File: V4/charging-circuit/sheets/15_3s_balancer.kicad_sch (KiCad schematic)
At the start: 29 parts, among them Q12 AO4892, Q13 BSS84, SW2 TS-1088R-02026, U16 NTC10K/0805/F, U20 BQ76920PW

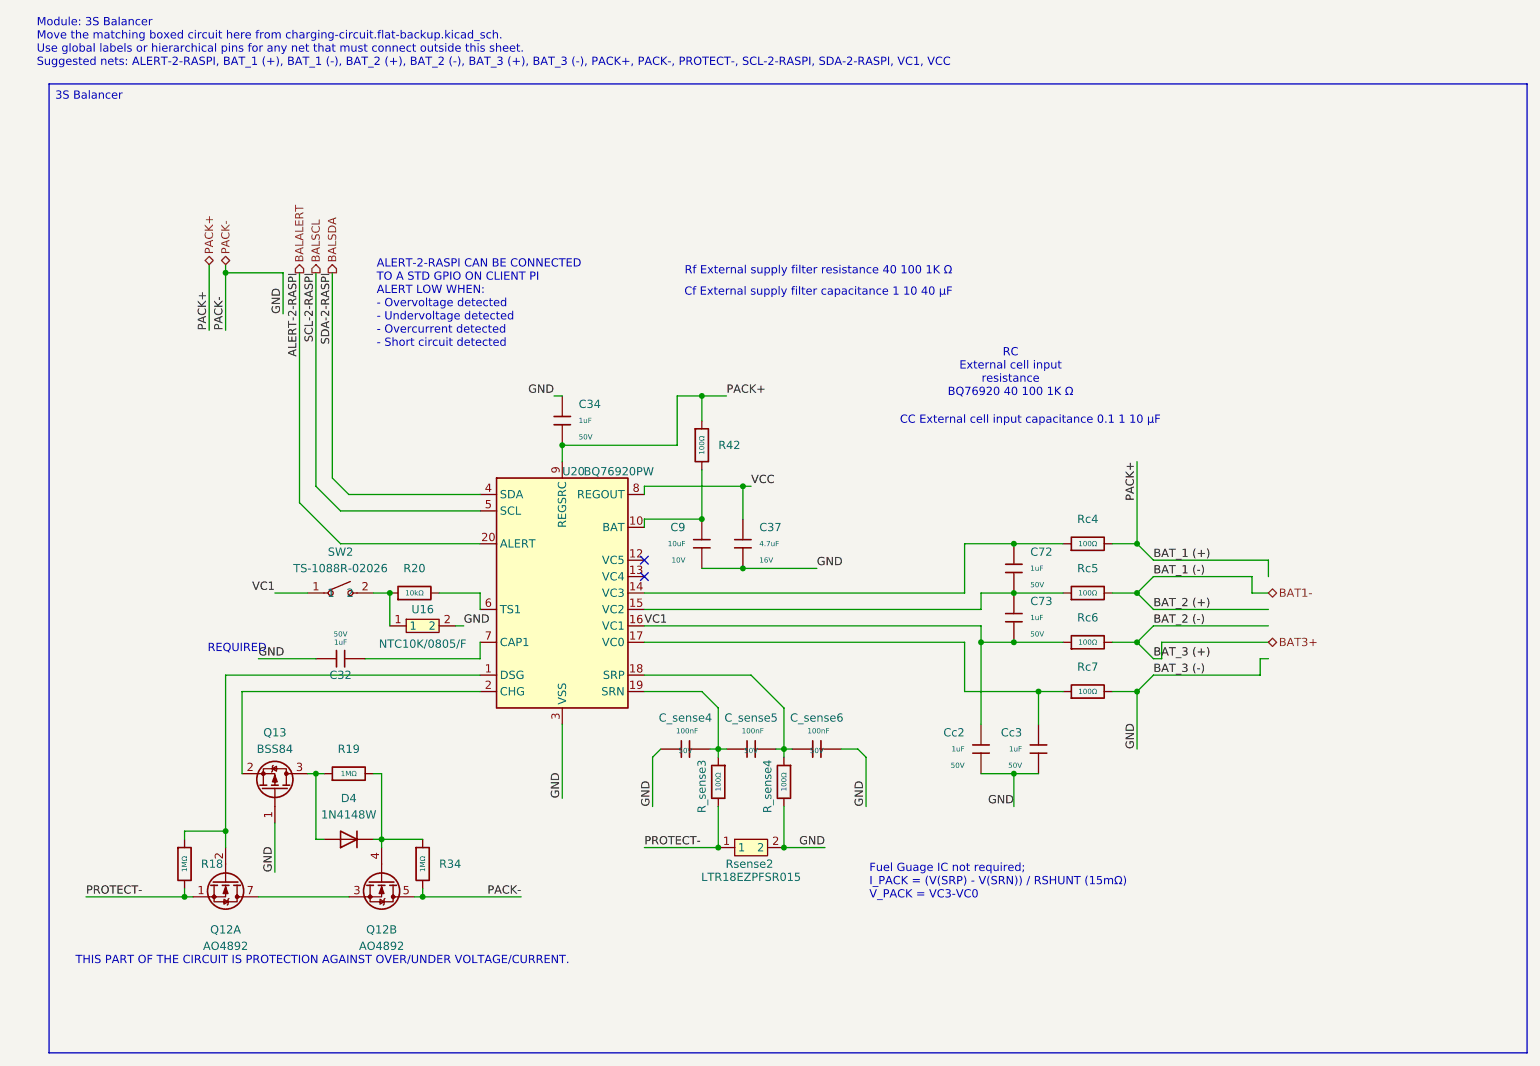
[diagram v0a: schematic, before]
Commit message: schem
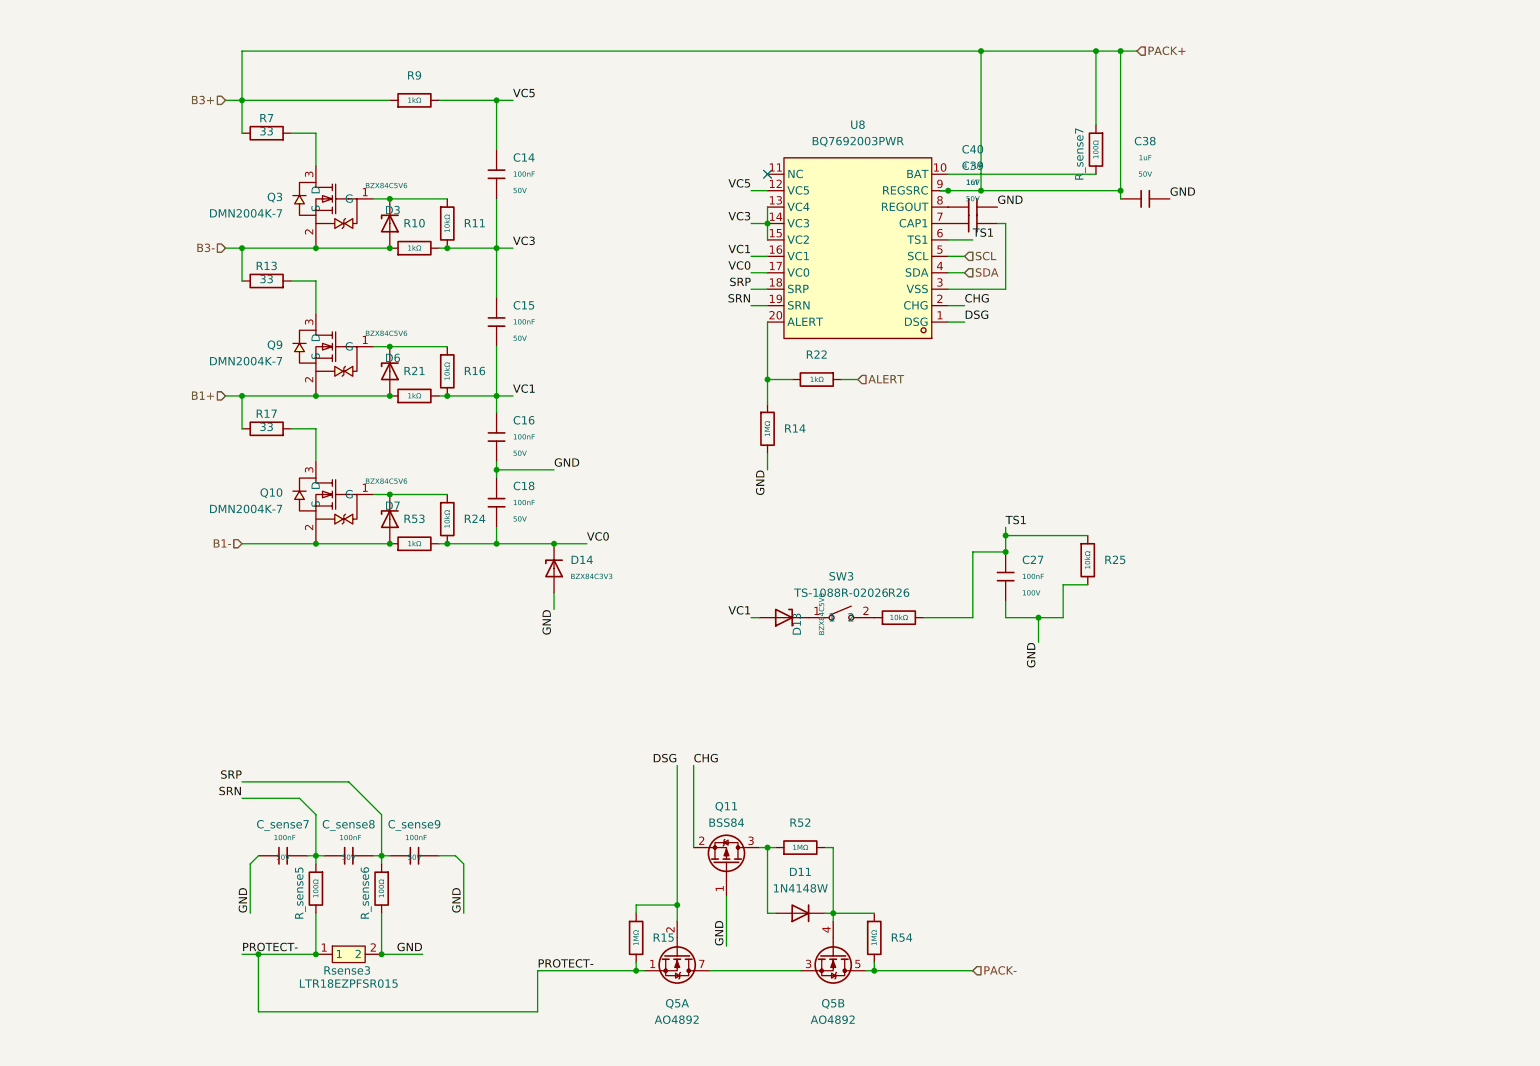
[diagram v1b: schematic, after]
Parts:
- removed C32: 1uF, PCM_JLCPCB:C_1206, symbol PCM_JLCPCB-Capacitors:1206,1uF
- removed C34, C72, C73, Cc2, Cc3: 1uF, PCM_JLCPCB:C_0603, symbol PCM_JLCPCB-Capacitors:0603,1uF
- removed C37: 4.7uF, PCM_JLCPCB:C_0603, symbol PCM_JLCPCB-Capacitors:0603,4.7uF
- removed C9: 10uF, PCM_JLCPCB:C_0603, symbol PCM_JLCPCB-Capacitors:0603,10uF
- removed C_sense4, C_sense5, C_sense6: 100nF, PCM_JLCPCB:C_0603, symbol PCM_JLCPCB-Capacitors:0603,100nF
- removed D4: 1N4148W, Diode_SMD:D_SOD-123, symbol Diode:1N4148W
- removed Q12: AO4892, Package_SO:SOIC-8_3.9x4.9mm_P1.27mm, symbol Transistor_FET:AO4892
- removed Q13: BSS84, Package_TO_SOT_SMD:SOT-23, symbol Transistor_FET:BSS84
- removed R18, R19, R34: 1MΩ, PCM_JLCPCB:R_0603, symbol PCM_JLCPCB-Resistors:0603,1MΩ
- removed R20: 10kΩ, PCM_JLCPCB:R_0603, symbol PCM_JLCPCB-Resistors:0603,10kΩ
- removed R42, R_sense3, R_sense4, Rc4, Rc5, Rc6, Rc7: 100Ω, PCM_JLCPCB:R_0603, symbol PCM_JLCPCB-Resistors:0603,100Ω
- removed Rsense2: LTR18EZPFSR015, easyeda2kicad:R0612, symbol easyeda2kicad:LTR18EZPFSR015
- removed SW2: TS-1088R-02026, easyeda2kicad:SW-SMD_L3.9-W3.0-P4.45, symbol easyeda2kicad:TS-1088R-02026
- removed U16: NTC10K/0805/F, easyeda2kicad:R0805, symbol easyeda2kicad:NTC10K_0805_F
- removed U20: BQ76920PW, Package_SO:TSSOP-20_4.4x6.5mm_P0.65mm, symbol Battery_Management:BQ76920PW
- added C14, C15, C16, C18, C_sense7, C_sense8, C_sense9: 100nF, PCM_JLCPCB:C_0603, symbol PCM_JLCPCB-Capacitors:0603,100nF
- added C27: 100nF, PCM_JLCPCB:C_0805, symbol PCM_JLCPCB-Capacitors:0805,100nF
- added C38, C39: 1uF, PCM_JLCPCB:C_0603, symbol PCM_JLCPCB-Capacitors:0603,1uF
- added C40: 4.7uF, PCM_JLCPCB:C_0603, symbol PCM_JLCPCB-Capacitors:0603,4.7uF
- added D11: 1N4148W, Diode_SMD:D_SOD-123, symbol Diode:1N4148W
- added D13, D3, D6, D7: BZX84C5V6, PCM_JLCPCB:D_SOT-23, symbol PCM_JLCPCB-Diodes:Zener,BZX84C5V6
- added D14: BZX84C3V3, PCM_JLCPCB:D_SOT-23, symbol PCM_JLCPCB-Diodes:Zener,BZX84C3V3
- added Q10, Q3, Q9: DMN2004K-7, EasyEDA:SOT-23-3_L3.0-W1.7-P0.95-LS2.9-BR, symbol EasyEDA:DMN2004K-7
- added Q11: BSS84, Package_TO_SOT_SMD:SOT-23, symbol Transistor_FET:BSS84
- added Q5: AO4892, Package_SO:SOIC-8_3.9x4.9mm_P1.27mm, symbol Transistor_FET:AO4892
- added R10, R21, R22, R53, R9: 1kΩ, PCM_JLCPCB:R_0805, symbol PCM_JLCPCB-Resistors:0805,1kΩ
- added R11, R16, R24, R25, R26: 10kΩ, PCM_JLCPCB:R_0805, symbol PCM_JLCPCB-Resistors:0805,10kΩ
- added R13, R17, R7: 33, symbol Device:R
- added R14: 1MΩ, PCM_JLCPCB:R_0805, symbol PCM_JLCPCB-Resistors:0805,1MΩ
- added R15, R52, R54: 1MΩ, PCM_JLCPCB:R_0603, symbol PCM_JLCPCB-Resistors:0603,1MΩ
- added R_sense5, R_sense6, R_sense7: 100Ω, PCM_JLCPCB:R_0603, symbol PCM_JLCPCB-Resistors:0603,100Ω
- added Rsense3: LTR18EZPFSR015, easyeda2kicad:R0612, symbol easyeda2kicad:LTR18EZPFSR015
- added SW3: TS-1088R-02026, easyeda2kicad:SW-SMD_L3.9-W3.0-P4.45, symbol easyeda2kicad:TS-1088R-02026
- added U8: BQ7692003PWR, EasyEDA:TSSOP-20_L6.5-W4.4-P0.65-LS6.4-BL, symbol EasyEDA:BQ7692003PWR
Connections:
- net PACK-: now also Q5.5 (D2), Q5.6 (D2), R54.2
- net PROTECT-: now also Q5.1 (S1), R15.2, R_sense5.2, Rsense3.1
- net VC1: now also C15.2, C16.1, D13.1, R16.2, R21.2, U8.16 (VC1)
- new net: C39.1, U8.7 (CAP1)
- new net: C39.2, U8.3 (VSS)
- new net: R_sense7.2, U8.10 (BAT)
- new net: D11.1 (K), Q5.4 (G2), R52.2, R54.1
- new net: D11.2 (A), Q11.3 (D), R52.1
- new net: D6.3, Q9.1 (G), R16.1
- new net: Q9.3 (D), R13.2
- new net: C40.1, U8.8 (REGOUT)
- new net: D3.3, Q3.1 (G), R11.1
- new net: Q3.3 (D), R7.2
- new net: Q10.3 (D), R17.2
- new net: D7.3, Q10.1 (G), R24.1
- new net: R14.1, R22.2, U8.20 (ALERT)
- new net: D13.3, SW3.1
- new net: R26.1, SW3.2
- new net: Q5.3 (S2), Q5.7 (D1), Q5.8 (D1)
- new net ALERT: R22.1
- new net B1+: D6.1, Q9.2 (S), R17.1, R21.1
- new net B1-: D7.1, Q10.2 (S), R53.1
- new net B3+: C38.1, R7.1, R9.1, R_sense7.1, U8.9 (REGSRC)
- new net B3-: D3.1, Q3.2 (S), R10.1, R13.1
- new net CHG: Q11.2 (S), U8.2 (CHG)
- new net DSG: Q5.2 (G1), R15.1, U8.1 (DSG)
- new net GND: C16.2, C18.1, C27.2, C38.2, C40.2, C_sense7.1, C_sense9.2, D14.1, Q11.1 (G), R14.2, R25.2, R_sense6.2, Rsense3.2
- new net SCL: U8.5 (SCL)
- new net SDA: U8.4 (SDA)
- new net SRN: C_sense7.2, C_sense8.1, R_sense5.1, U8.19 (SRN)
- new net SRP: C_sense8.2, C_sense9.1, R_sense6.1, U8.18 (SRP)
- new net TS1: C27.1, R25.1, R26.2, U8.6 (TS1)
- new net VC0: C18.2, D14.3, R24.2, R53.2, U8.17 (VC0)
- new net VC3: C14.2, C15.1, R10.2, R11.2, U8.13 (VC4), U8.14 (VC3), U8.15 (VC2)
- new net VC5: C14.1, R9.2, U8.12 (VC5)
- no-connect marks 2 -> 1
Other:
- note removed: "ALERT-2-RASPI CAN BE CONNECTED TO A STD GPIO ON CLIENT PI ALERT LOW WHEN: - Overvoltage detected - Undervoltage detected - Overcurrent detected - Short circuit detected"
- note removed: "CC External cell input capacitance 0.1 1 10 µF"
- note removed: "Cf External supply filter capacitance 1 10 40 µF"
- note removed: "Fuel Guage IC not required; I_PACK = (V(SRP) - V(SRN)) / RSHUNT (15mΩ) V_PACK = VC3-VC0"
- note removed: "Module: 3S Balancer Move the matching boxed circuit here from charging-circuit.flat-backup.kicad_sch. Use global labels or hierarchical pins for any net that must connect outside this sheet. Suggested nets: ALERT-2-RASPI, BAT_1 (+), BAT_1 (-), BAT_2 (+), BAT_2 (-), BAT_3 (+), BAT_3 (-), PACK+, PACK-, PROTECT-, SCL-2-RASPI, SDA-2-RASPI, VC1, VCC"
- note removed: "RC External cell input resistance BQ76920 40 100 1K Ω"
- note removed: "REQUIRED"
- note removed: "Rf External supply filter resistance 40 100 1K Ω"
- note removed: "THIS PART OF THE CIRCUIT IS PROTECTION AGAINST OVER/UNDER VOLTAGE/CURRENT."

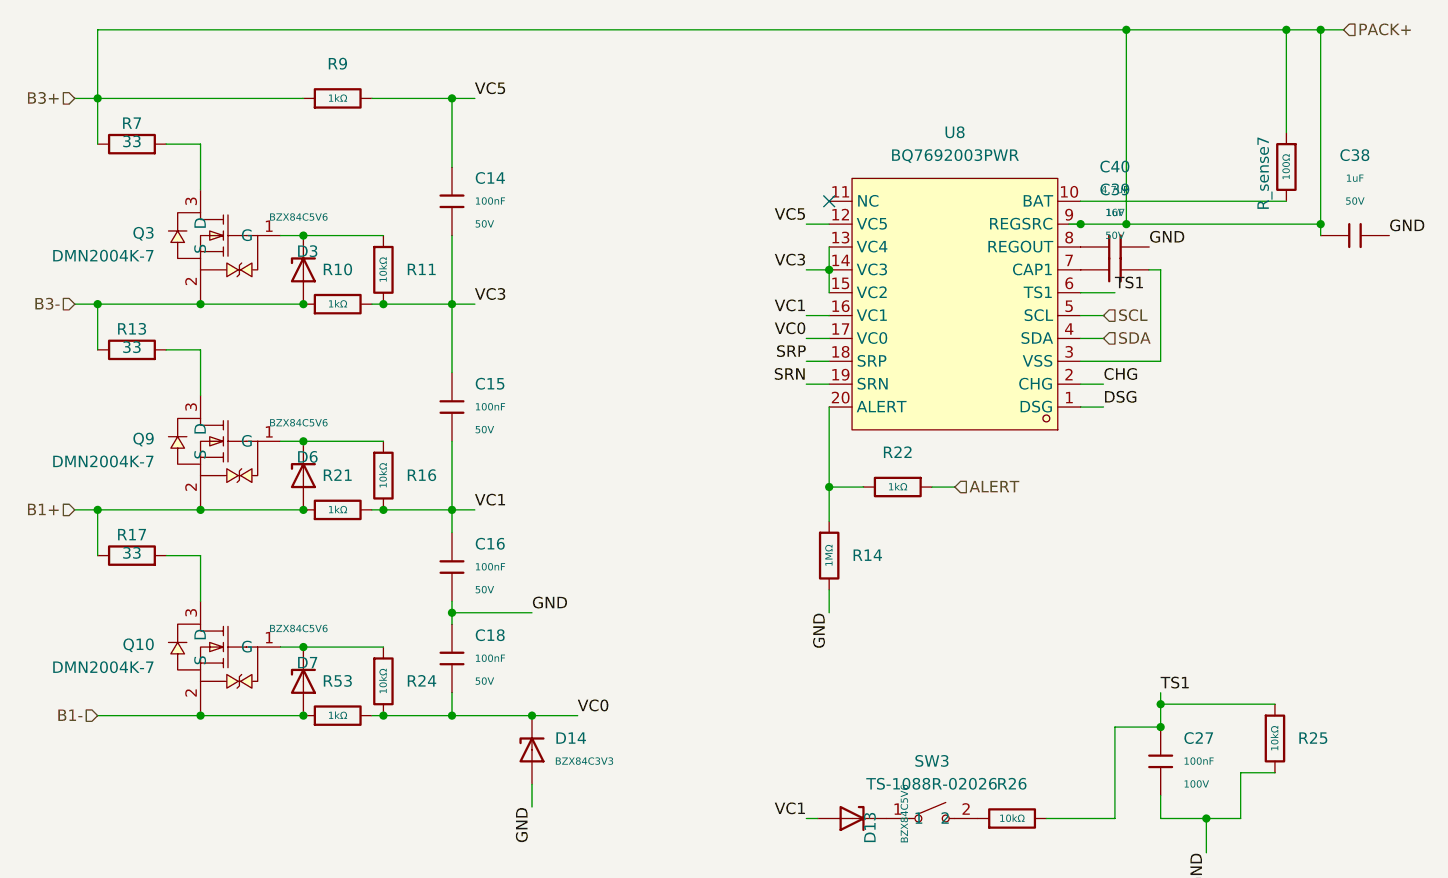
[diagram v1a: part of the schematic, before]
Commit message: sunday
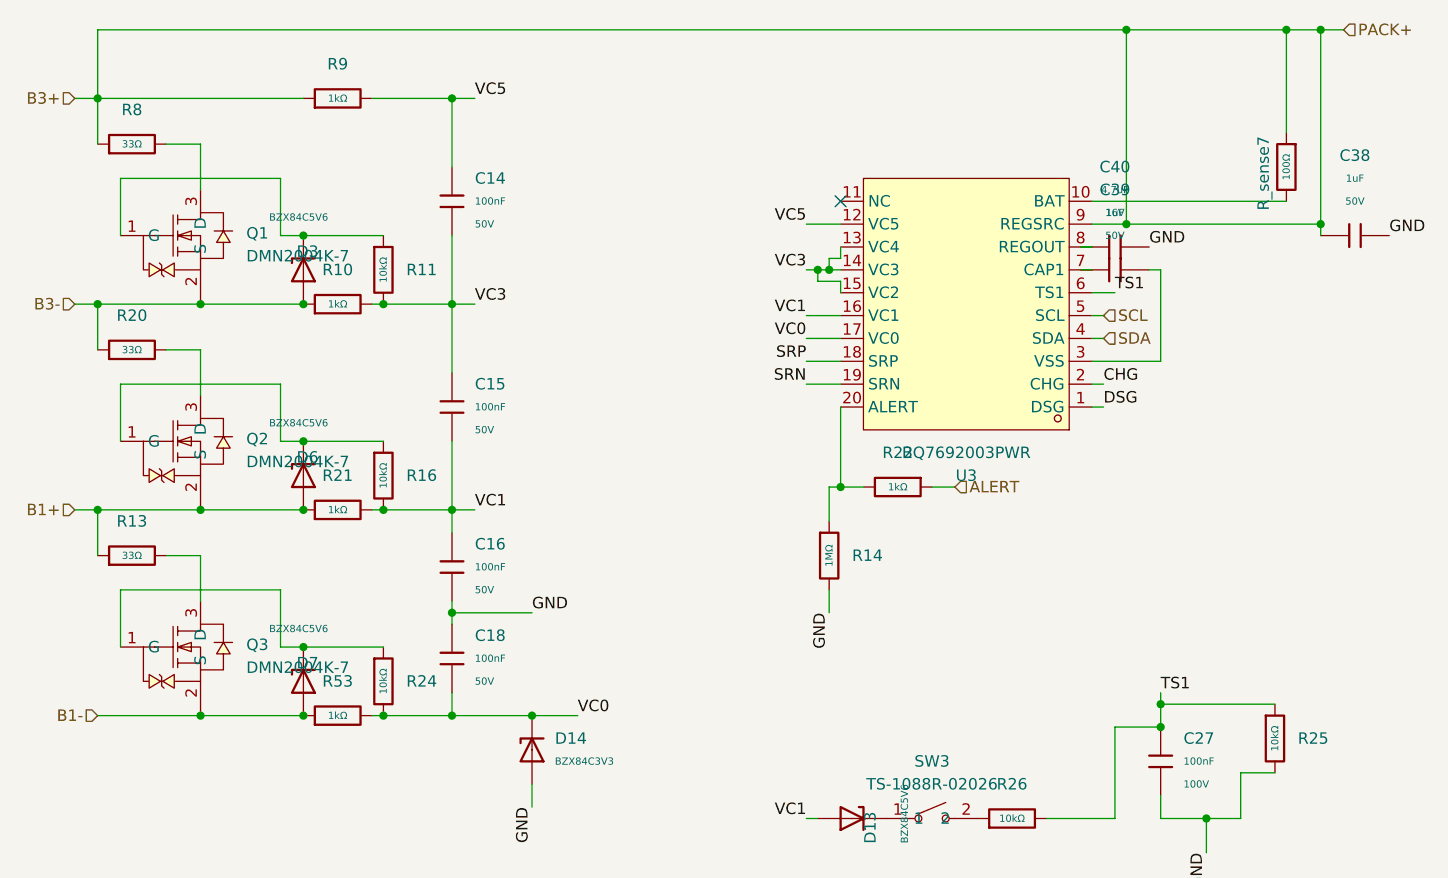
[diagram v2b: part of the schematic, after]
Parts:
- removed Q10, Q3, Q9: DMN2004K-7, EasyEDA:SOT-23-3_L3.0-W1.7-P0.95-LS2.9-BR, symbol EasyEDA:DMN2004K-7
- removed R13, R17, R7: 33, symbol Device:R
- removed U8: BQ7692003PWR, EasyEDA:TSSOP-20_L6.5-W4.4-P0.65-LS6.4-BL, symbol EasyEDA:BQ7692003PWR
- added Q1, Q2, Q3: DMN2004K-7, easyeda2kicad:SOT-23-3_L3.0-W1.7-P0.95-LS2.9-BR, symbol easyeda2kicad:DMN2004K-7
- added R13, R20, R8: 33Ω, PCM_JLCPCB:R_0805, symbol PCM_JLCPCB-Resistors:0805,33Ω
- added U3: BQ7692003PWR, easyeda2kicad:TSSOP-20_L6.5-W4.4-P0.65-LS6.4-BL, symbol easyeda2kicad:BQ7692003PWR
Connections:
- net B1+: now also Q2.2 (S), R13.1
- net B1-: now also Q3.2 (S)
- net B3+: now also R8.1, U3.9 (REGSRC)
- net B3-: now also Q1.2 (S), R20.1
- net CHG: now also U3.2 (CHG)
- net DSG: now also U3.1 (DSG)
- net SCL: now also U3.5 (SCL)
- net SDA: now also U3.4 (SDA)
- net SRN: now also U3.19 (SRN)
- net SRP: now also U3.18 (SRP)
- net TS1: now also U3.6 (TS1)
- net VC0: now also U3.17 (VC0)
- net VC1: now also U3.16 (VC1)
- net VC3: now also U3.13 (VC4), U3.14 (VC3), U3.15 (VC2)
- net VC5: now also U3.12 (VC5)
- net at C39.1: now also U3.7 (CAP1)
- net at C39.2: now also U3.3 (VSS)
- net at R_sense7.2: now also U3.10 (BAT)
- net at D6.3, R16.1: now also Q2.1 (G)
- net at C40.1: now also U3.8 (REGOUT)
- net at D3.3, R11.1: now also Q1.1 (G)
- net at D7.3, R24.1: now also Q3.1 (G)
- net at R14.1, R22.2: now also U3.20 (ALERT)
- new net: Q3.3 (D), R13.2
- new net: Q2.3 (D), R20.2
- new net: Q1.3 (D), R8.2
